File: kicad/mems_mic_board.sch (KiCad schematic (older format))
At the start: 8 parts, among them J1 Conn_01x08_Male, J2 Conn_01x06_Male, J3 Conn_01x01_Male, J4 Conn_01x10_Male, J5 Conn_01x08_Male, U1 tactile_sw, U2 mems_mic, U3 mems_mic

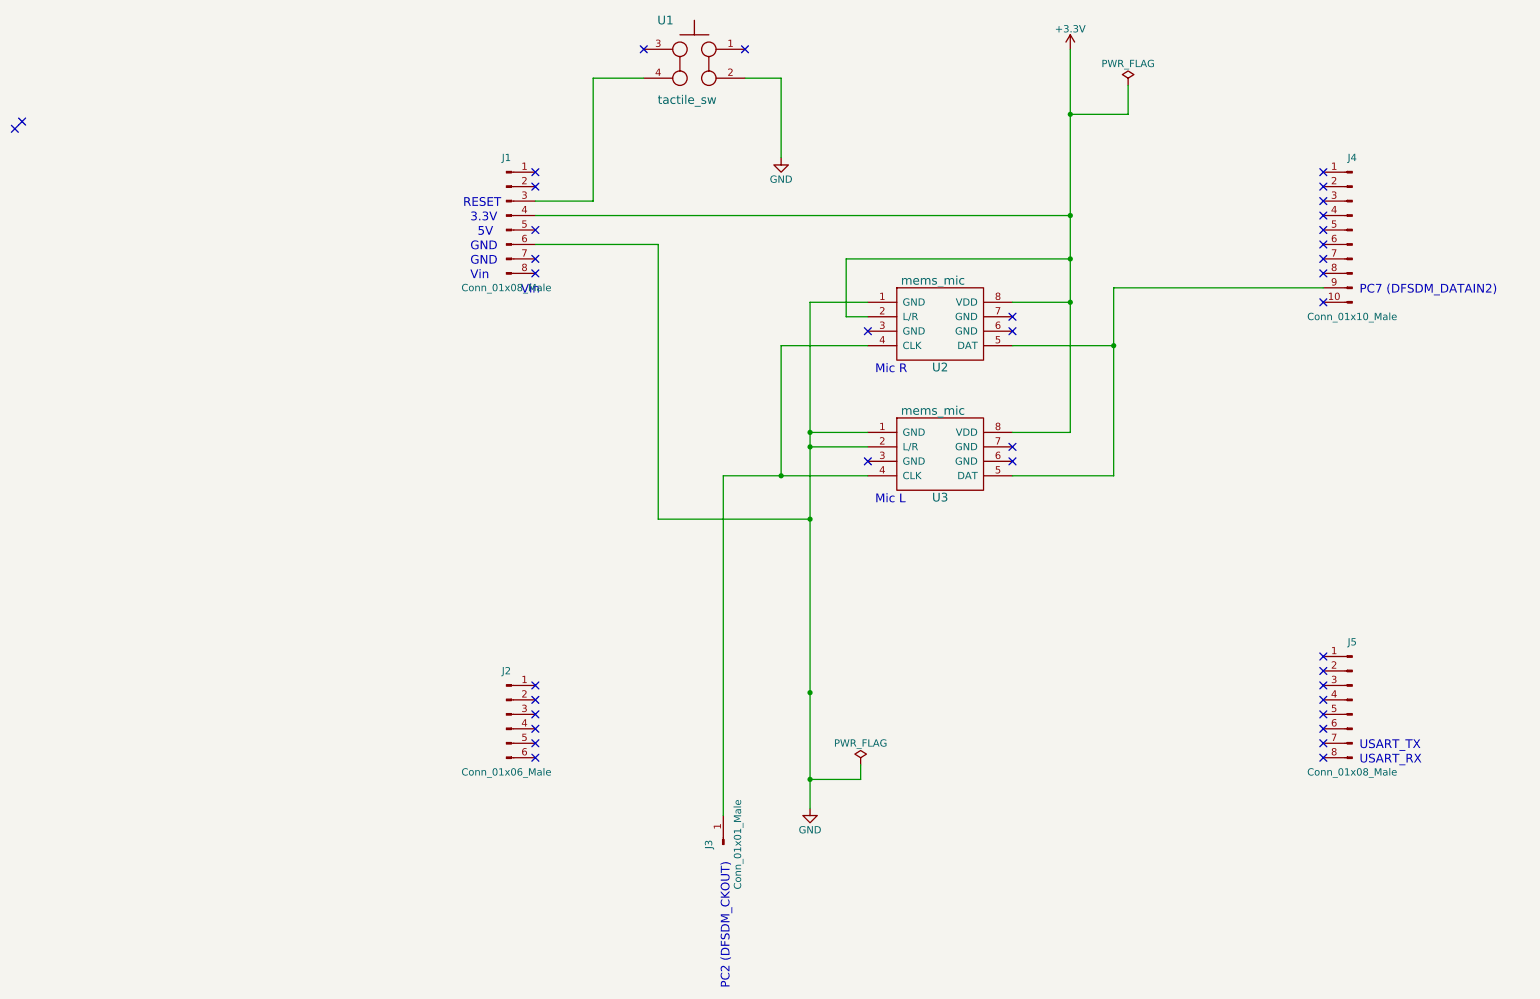
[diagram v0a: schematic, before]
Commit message: update
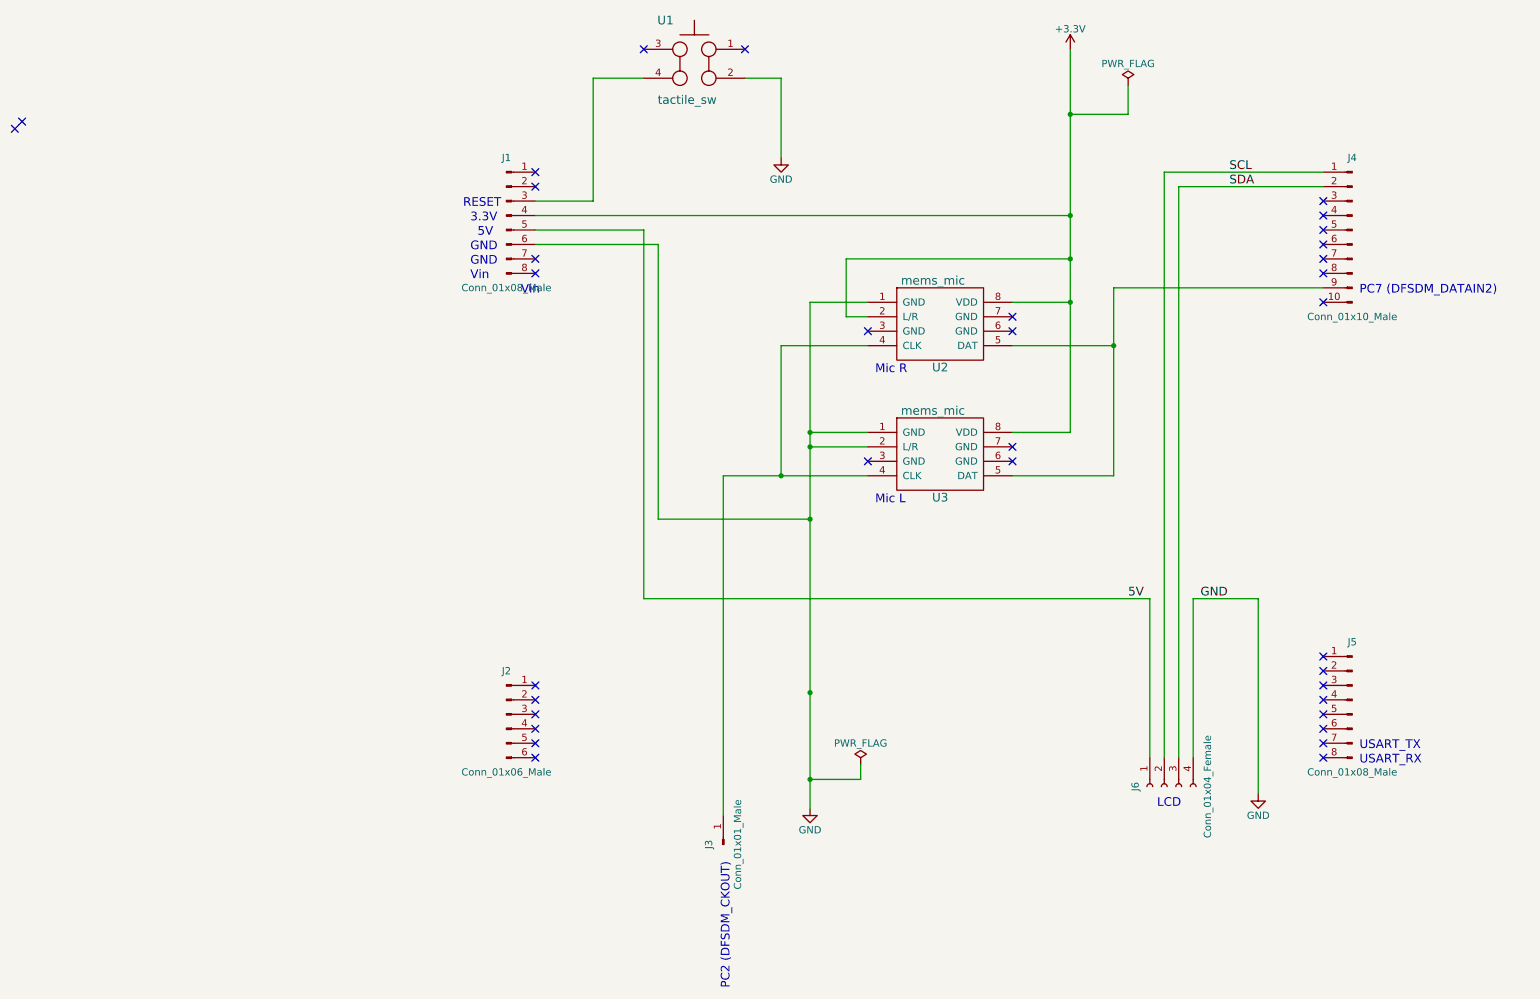
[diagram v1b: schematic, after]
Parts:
- added J6: Conn_01x04_Female, mcu:pin-socket-4p, symbol Conn_01x04_Female
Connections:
- net GND: now also J6.4 (Pin_4)
- net 5V: now reaches J1.5 (Pin_5)
- net 5V: now also J6.1 (Pin_1)
- net SCL: now reaches J4.1 (Pin_1)
- net SCL: now also J6.2 (Pin_2)
- net SDA: now reaches J4.2 (Pin_2)
- net SDA: now also J6.3 (Pin_3)
- no-connect marks 38 -> 35
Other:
- note added: "LCD"
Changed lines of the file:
@@
 NoConn ~ 8050 5750
 NoConn ~ 8050 5850
-NoConn ~ 2600 2200
 $Comp
 L Conn_01x08_Male J1
@@
 	-1   0    0    -1
 $EndComp
-NoConn ~ 8050 1900
-NoConn ~ 8050 1800
 NoConn ~ 3350 950
 NoConn ~ 4050 950
+$Comp
+L Conn_01x04_Female J6
+U 1 1 5C792525
+P 6950 6050
+F 0 "J6" H 6950 6250 50  0000 C CNN
+F 1 "Conn_01x04_Female" H 6950 5750 50  0000 C CNN
+F 2 "mcu:pin-socket-4p" H 6950 6050 50  0001 C CNN
+F 3 "" H 6950 6050 50  0001 C CNN
+	1    6950 6050
+	0    -1   1    0
+$EndComp
+Wire Wire Line
+	8050 1800 6950 1800
+Wire Wire Line
+	6950 1800 6950 5850
+Wire Wire Line
+	8050 1900 7050 1900
+Wire Wire Line
+	7050 1900 7050 5850
+Wire Wire Line
+	2600 2200 3350 2200
+Wire Wire Line
+	3350 2200 3350 4750
+Wire Wire Line
+	3350 4750 6850 4750
+Wire Wire Line
+	6850 4750 6850 5850
+$Comp
+L GND #PWR06
+U 1 1 5C79271E
+P 7600 6100
+F 0 "#PWR06" H 7600 5850 50  0001 C CNN
+F 1 "GND" H 7600 5950 50  0000 C CNN
+F 2 "" H 7600 6100 50  0001 C CNN
+F 3 "" H 7600 6100 50  0001 C CNN
+	1    7600 6100
+	1    0    0    -1
+$EndComp
+Wire Wire Line
+	7150 5850 7150 4750
+Wire Wire Line
+	7150 4750 7600 4750
+Wire Wire Line
+	7600 4750 7600 6100
+Text Label 7400 1800 0    60   ~ 0
+SCL
+Text Label 7400 1900 0    60   ~ 0
+SDA
+Text Label 6700 4750 0    60   ~ 0
+5V
+Text Label 7200 4750 0    60   ~ 0
+GND
+Text Notes 6900 6200 0    60   ~ 0
+LCD
 $EndSCHEMATC
